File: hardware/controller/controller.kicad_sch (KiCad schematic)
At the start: 4 parts, among them U1 ZX-PM2.54-1-16PY, U2 ZX-PM2.54-1-16PY, U3 ZX-PM2.54-1-16PY, U4 ZX-PM2.54-1-16PY

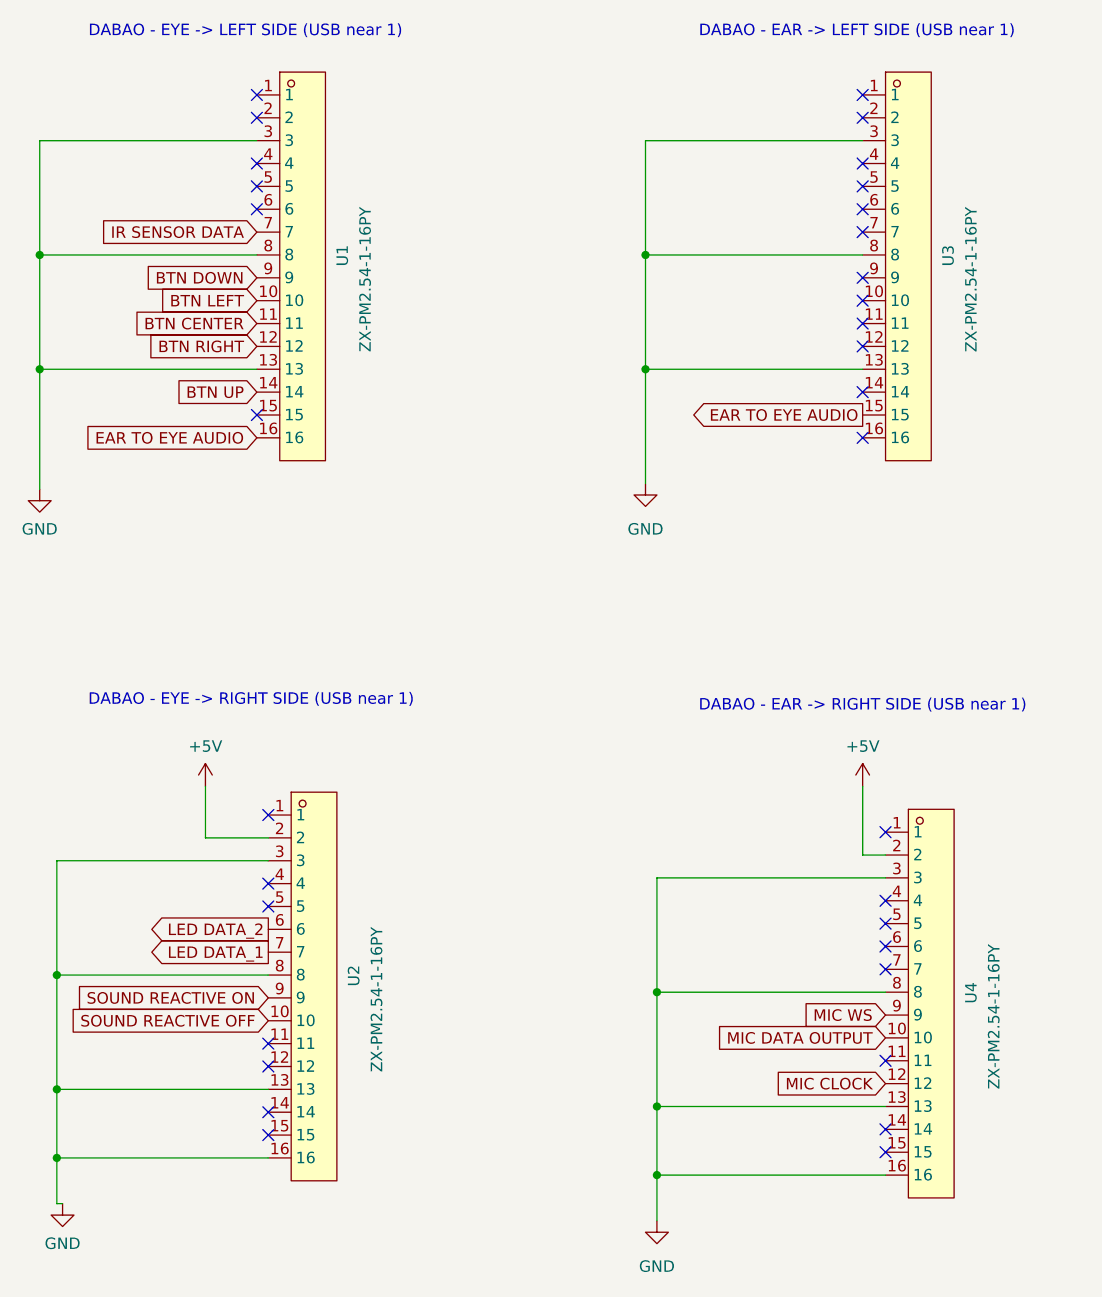
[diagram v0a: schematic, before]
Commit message: feedback on the controller
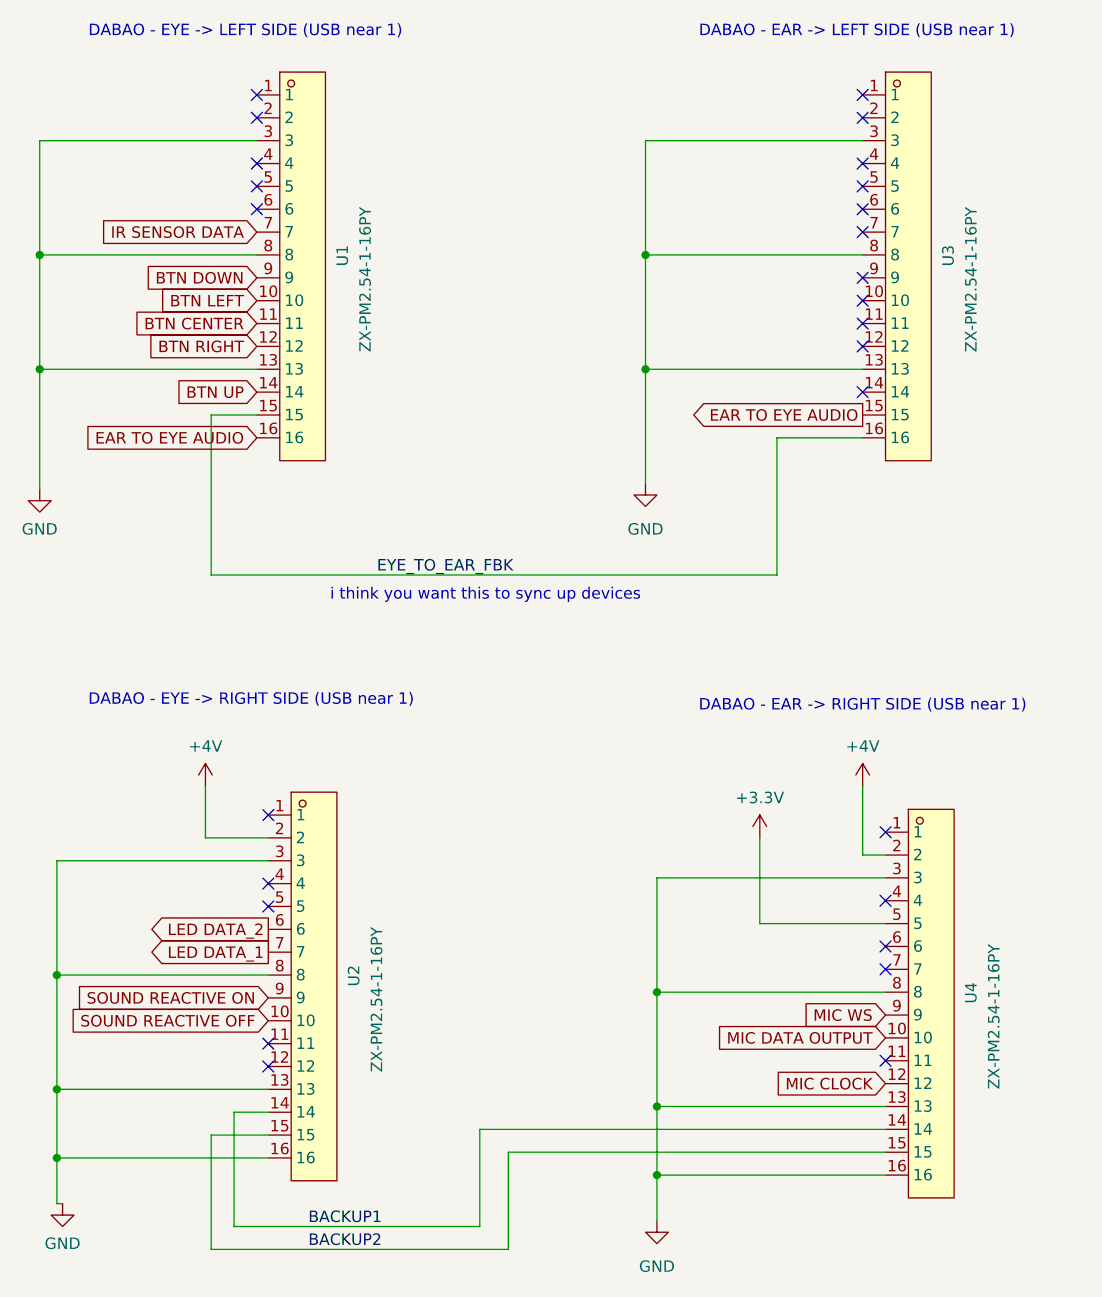
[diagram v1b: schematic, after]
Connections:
- net BACKUP1: now reaches U2.14
- net BACKUP1: now also U4.14
- net BACKUP2: now reaches U2.15
- net BACKUP2: now also U4.15
- net EYE_TO_EAR_FBK: now reaches U3.16
- net EYE_TO_EAR_FBK: now also U1.15
- net +3.3V: now reaches U4.5
- net +5V renamed +4V
- no-connect marks 33 -> 26
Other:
- note added: "i think you want this to sync up devices"
